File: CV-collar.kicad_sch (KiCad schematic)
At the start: 42 parts, among them J2 MLX90614, J3 UART, J4 BATT_IN, J8 MTHR_I2C, J9 DTR_I2C, Q1 IRLML6401, Q2 AO3401A, SW1 BOOT, SW2 EN, SW3 Addr_SW, SW4 Debug_SW, SW5 PWR, U1 ESP32-WROOM-32, U2 MPU-6050, U3 DS3231M, U4 TPS63900, U5 CW2015CHBD

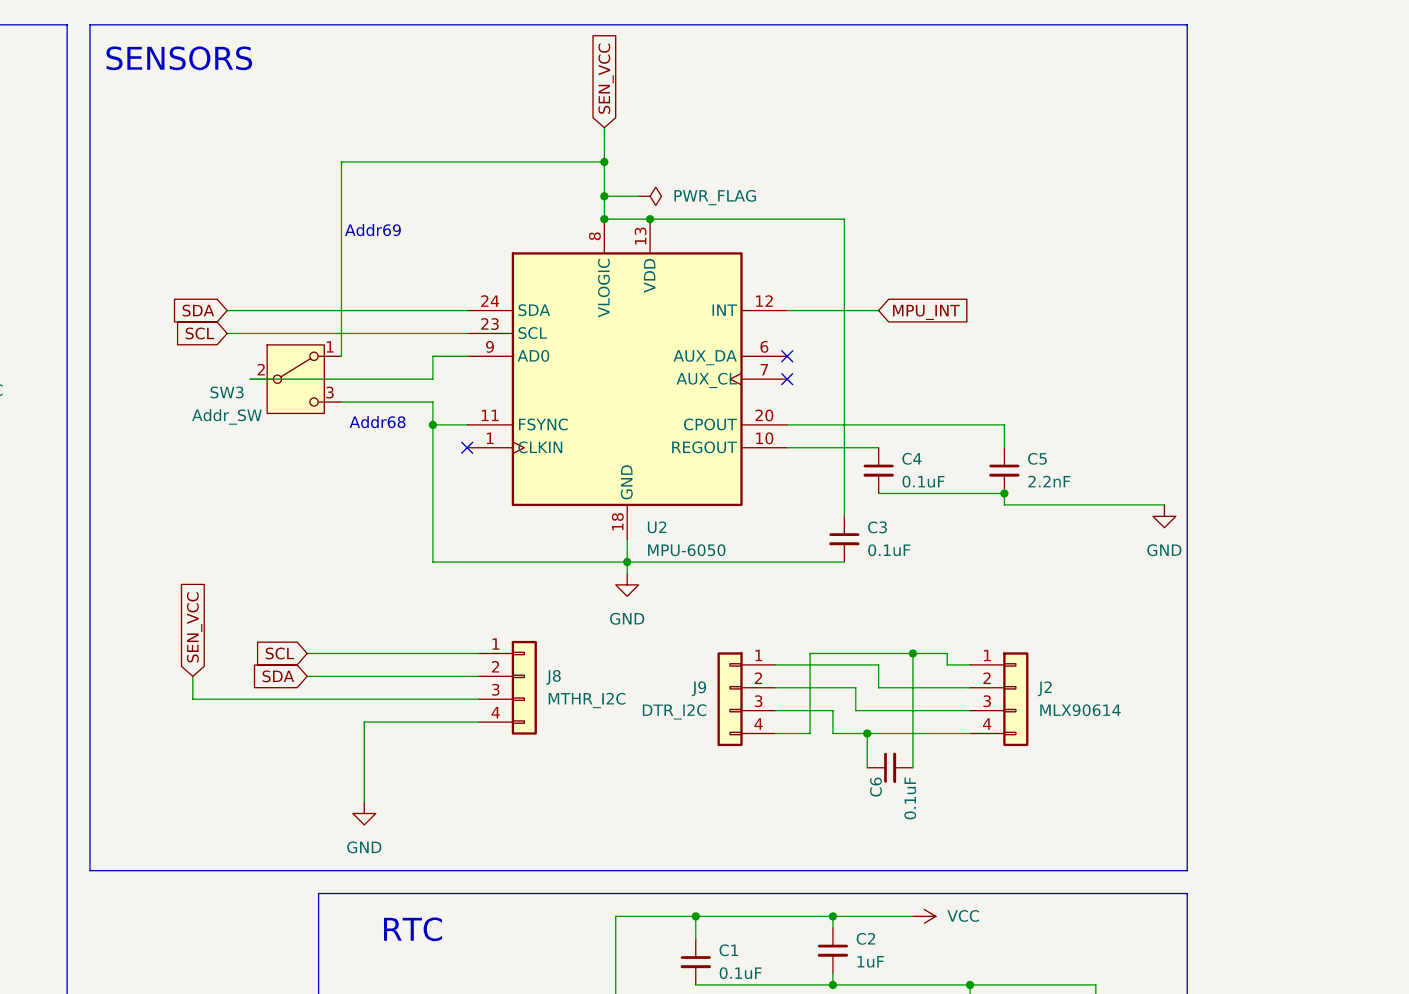
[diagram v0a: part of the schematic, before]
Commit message: latest before changing to more cost effective design
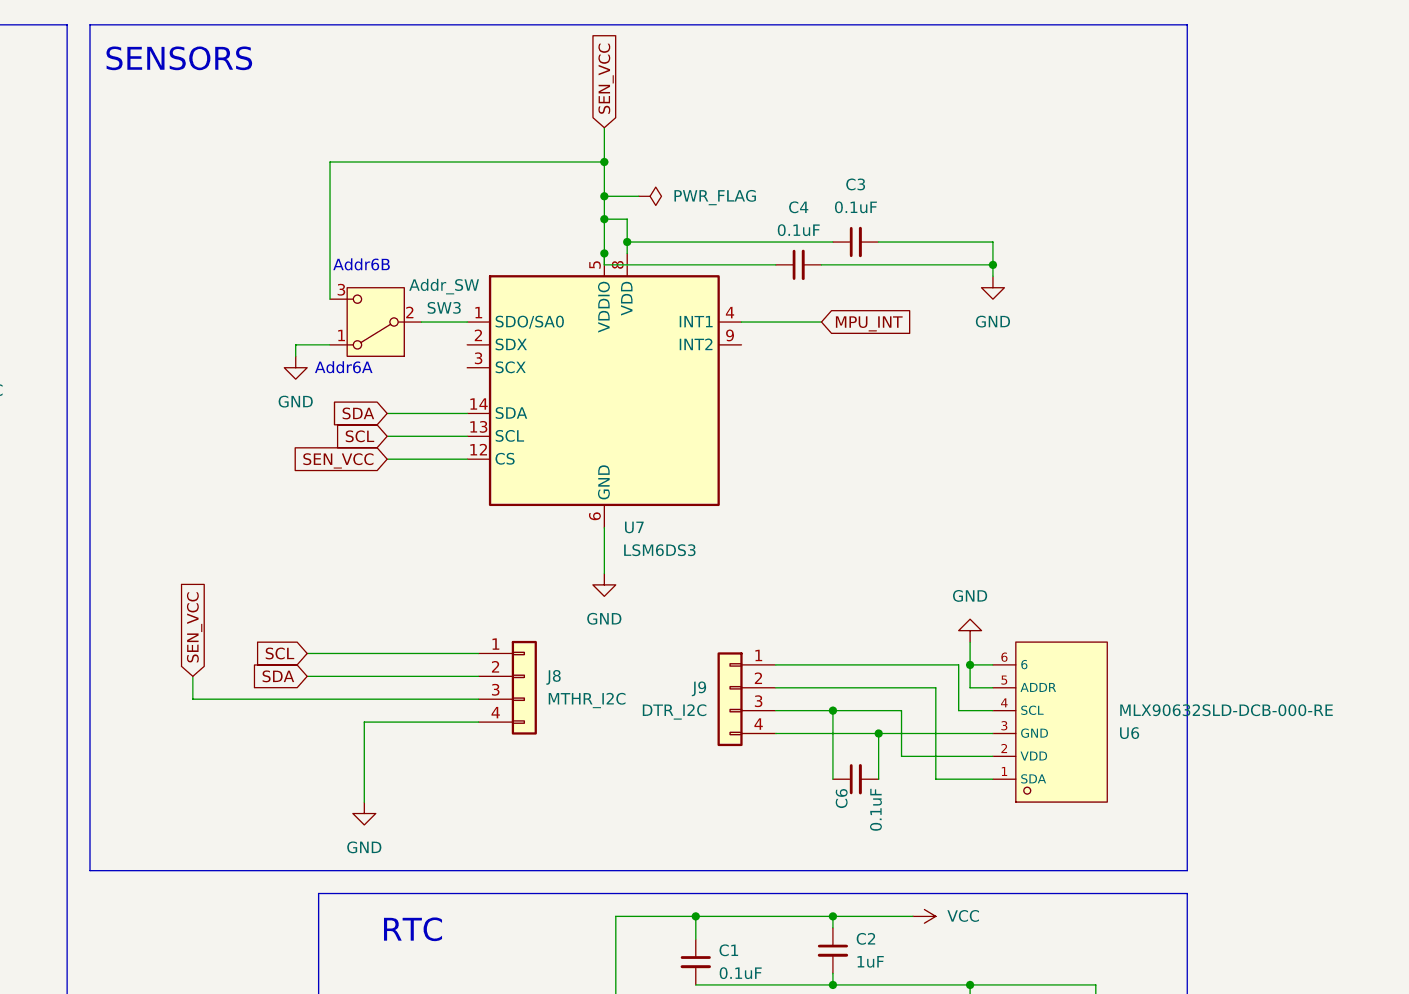
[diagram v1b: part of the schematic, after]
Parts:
- removed C5: 2.2nF, Capacitor_SMD:C_0603_1608Metric, symbol Device:C_Small
- removed J2: MLX90614, Package_TO_SOT_THT:TO-39-4_Window, symbol Connector_Generic:Conn_01x04
- removed U2: MPU-6050, Sensor_Motion:InvenSense_QFN-24_4x4mm_P0.5mm, symbol Sensor_Motion:MPU-6050
- added U6: MLX90632SLD-DCB-000-RE, footprint:SENSOR-SMD_MLX90632, symbol MLX90632SLD-DCB-000-RE:MLX90632SLD-DCB-000-RE
- added U7: LSM6DS3, Package_LGA:LGA-14_3x2.5mm_P0.5mm_LayoutBorder3x4y, symbol Sensor_Motion:LSM6DS3
- BT1: footprint Battery:BatteryHolder_Keystone_103_1x20mm -> Battery:BatteryHolder_Keystone_1060_1x2032; LCSC Part # C3038670 -> C70377
- U3: footprint Package_SO:SOIC-16W_7.5x10.3mm_P1.27mm -> Package_SO:SOIC-8_3.9x4.9mm_P1.27mm; LCSC Part # C37663 -> C107410
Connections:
- net GND: now also SW3.1 (A), U6.5 (ADDR), U6.6, U7.6 (GND), U7.7 (GND); no longer SW3.3 (C)
- net MPU_INT: now also U7.4 (INT1)
- net SCL: now also U7.13 (SCL)
- net SDA: now also U7.14 (SDA)
- net SEN_VCC: now also C4.1, SW3.3 (C), U7.12 (CS), U7.5 (VDDIO), U7.8 (VDD); no longer SW3.1 (A)
- net at SW3.2 (B): now also U7.1 (SDO/SA0)
- net at C6.2, J9.4 (Pin_4): now also U6.3 (GND)
- net at J9.1 (Pin_1): now also U6.4 (SCL)
- net at J9.2 (Pin_2): now also U6.1 (SDA)
- net at C6.1, J9.3 (Pin_3): now also U6.2 (VDD)
- no-connect marks 31 -> 28
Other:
- note added: "Addr6A"
- note added: "Addr6B"
- note removed: "Addr68"
- note removed: "Addr69"
- moved on the sheet: C3, C4, C6, SW3
